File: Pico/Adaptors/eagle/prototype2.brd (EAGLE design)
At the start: 45.8 x 20.7 mm, 13 parts, among them J1 JST-2P-SMD-PW-3410050P1

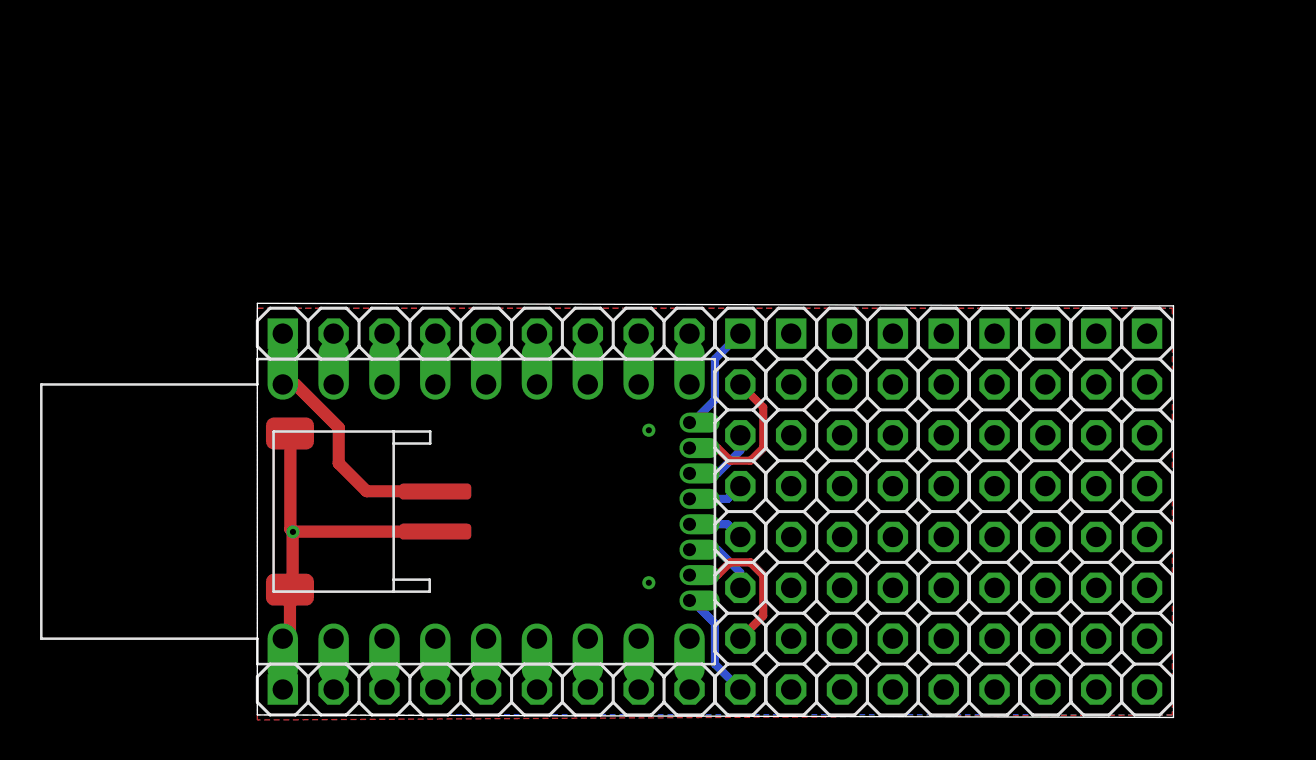
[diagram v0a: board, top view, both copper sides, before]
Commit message: a full panel
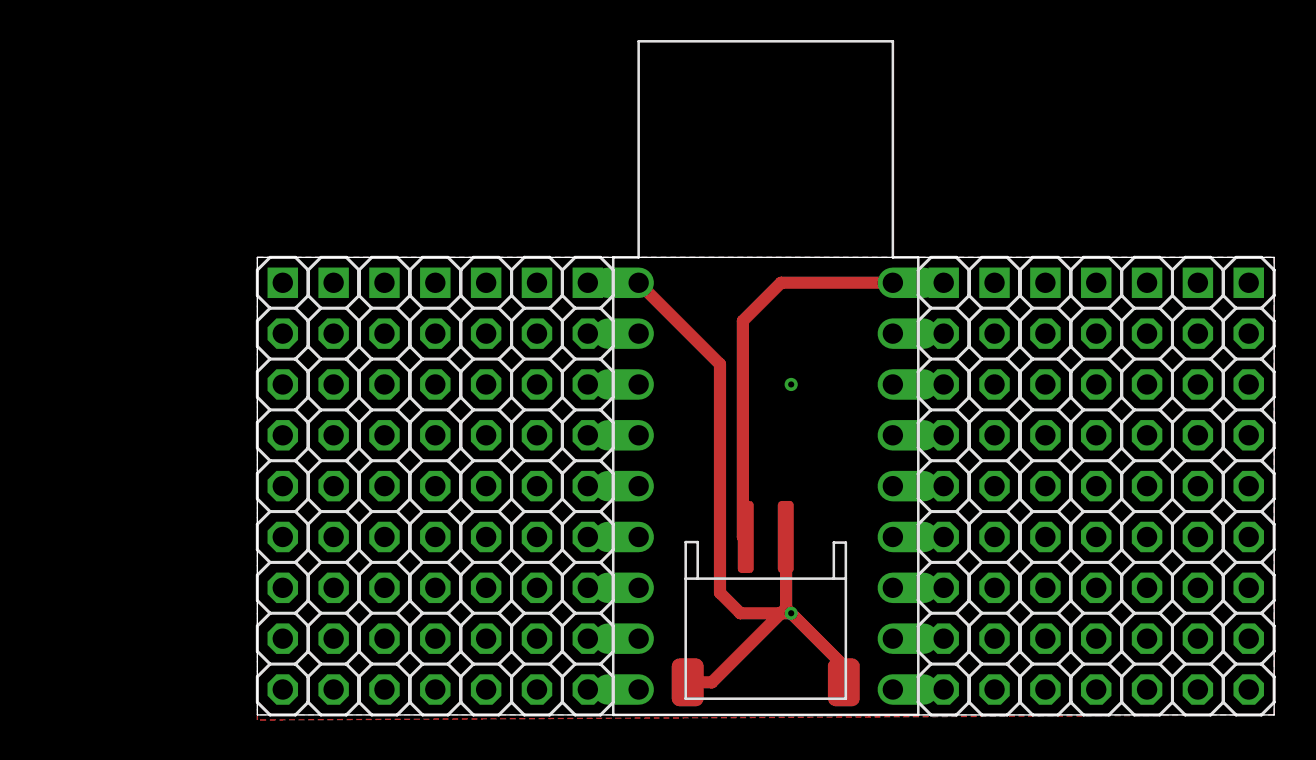
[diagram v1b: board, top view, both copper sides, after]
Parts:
- added JP12, JP13, JP14: (no value), pinhead-2:1X09-S
- JP1, JP10, JP11, JP2, JP5, JP6, JP7, JP8, JP9: device pinhead-2:1X08-S -> pinhead-2:1X09-S
- U$1: value ESPRUINO_PICO_SMD -> ESPRUINO_PICO_0.1; device espruino_pico:ESPRUINO_PICO_SMD -> espruino_pico:ESPRUINO_PICO_0.1
- moved JP1 25.4 mm to (1.27, 11.4)
- moved JP5 25.4 mm to (3.81, 11.4)
- moved JP6 25.4 mm to (6.35, 11.4)
- moved JP7 25.4 mm to (8.89, 11.4)
- moved JP8 25.4 mm to (11.4, 11.4)
- moved JP9 25.4 mm to (14.0, 11.4)
- moved JP3 24.1 mm to (34.3, 11.4), turned to 270 degrees
- moved J1 22.5 mm to (25.4, 3.81), turned to 0 degrees
- moved JP2 12.8 mm to (36.8, 11.4)
- moved JP4 11.4 mm to (16.5, 11.4), turned to 270 degrees
- moved U$1 10.2 mm to (25.4, 8.89), turned to 270 degrees
- moved JP11 2.84 mm to (41.9, 11.4)
- moved JP10 2.84 mm to (39.4, 11.4)
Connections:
- removed net N$1: JP2.2, U$1.A3
- removed net N$2: JP2.3, U$1.A2
- removed net N$24: JP2.1, U$1.A4
- removed net N$3: JP2.4, U$1.A1
- removed net N$4: JP2.5, U$1.A0
- removed net N$5: JP2.6, U$1.A10
- removed net N$6: JP2.7, U$1.B9
- removed net N$9: JP2.8, U$1.B8
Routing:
- net GND: track 20.2 -> 38.6 mm, vias 3 -> 2
- net N$15: track 13.4 -> 21.8 mm
- net N$1: track 7.86 -> 0.00 mm
- net N$6: track 7.86 -> 0.00 mm
- net N$9: track 5.57 -> 0.00 mm
- net N$24: track 5.57 -> 0.00 mm
- net N$5: track 3.78 -> 0.00 mm
- net N$2: track 3.78 -> 0.00 mm
- net N$4: track 2.80 -> 0.00 mm
- net N$3: track 2.80 -> 0.00 mm
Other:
- board size 45.8 x 20.7 mm -> 50.8 x 22.9 mm
